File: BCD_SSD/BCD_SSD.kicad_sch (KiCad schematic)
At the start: 25 parts, among them J1 Conn_01x06, J2 Conn_01x07, U1 Inverter, U10 AND-3, U11 AND-3, U12 AND-3, U13 AND-3, U14 AND-4, U15 OR, U16 OR-3, U17 OR, U18 AND, U19 AND, U2 Inverter, U20 AND-3, U21 OR, U22 OR-3, U3 Inverter, U39 AND, U4 Inverter, U5 AND-4, U6 AND-3, U7 OR, U8 AND-3, U9 AND-3

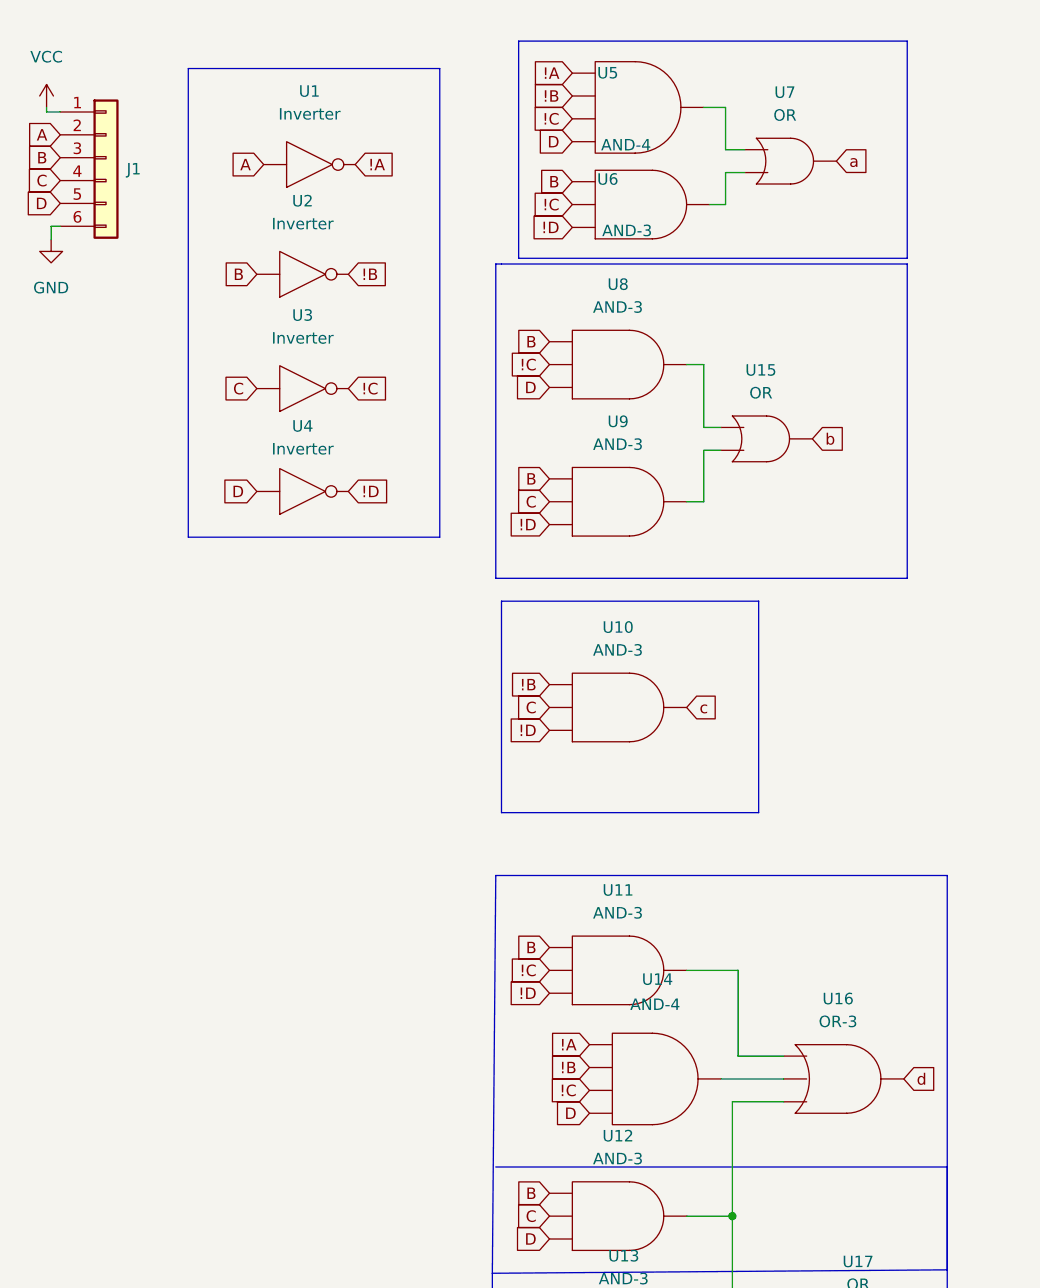
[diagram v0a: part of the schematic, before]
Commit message: Theoretically correct decoder
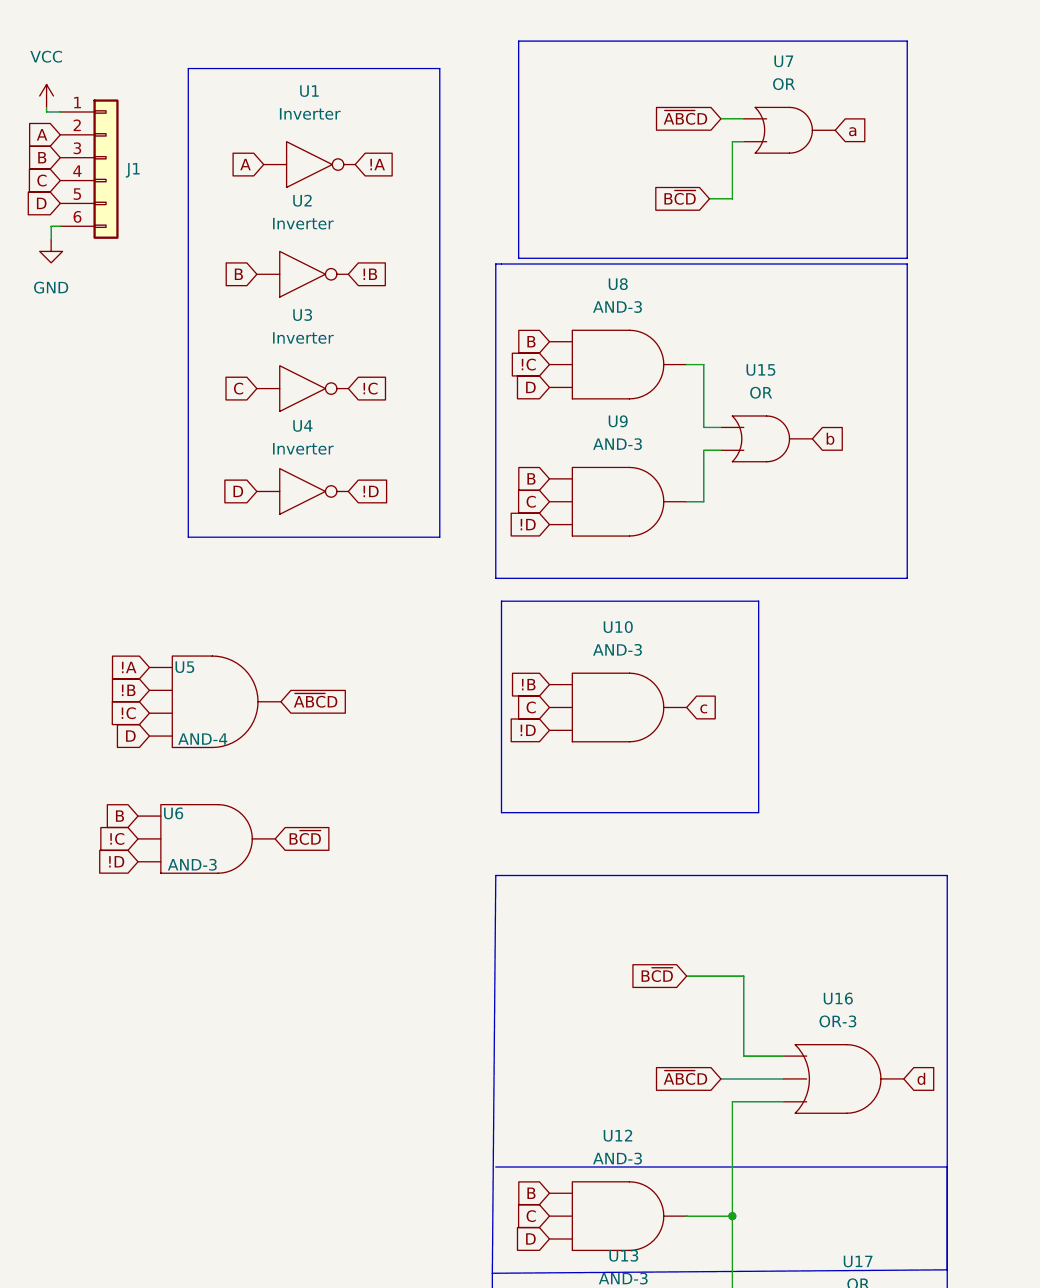
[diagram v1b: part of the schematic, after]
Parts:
- removed U11: AND-3, symbol AOI_Symbols:AND-3
- removed U14: AND-4, symbol AOI_Symbols:AND-4
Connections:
- net ~{ABC}D: now reaches U16.
- net ~{ABC}D: now also U5., U7.
- net B~{CD}: now reaches U6., U7.
- net B~{CD}: now also U16.
- new net: U15., U9.
- new net: U15., U8.
- new net: U12., U16., U17.
- new net: U13., U17.
- new net: U19., U21.
- new net: U18., U22.
- new net: U20., U22.
- new net: U22., U39.
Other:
- moved on the sheet: U7
